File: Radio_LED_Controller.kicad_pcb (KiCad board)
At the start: 2 copper layers, 21.5 x 12.5 mm, 17 parts, among them J1 Conn_01x04_Pin, J2 Conn_01x03_Pin, J3 Conn_01x05, J4 UPDI, J5 Conn_01x02_Pin, J6 Conn_01x02_Pin, J7 Conn_01x05, J8 Conn_01x03_Pin, J9 Conn_01x03_Pin, Q2 SS8050, Q3 SS8050, U1 ATtiny816-M

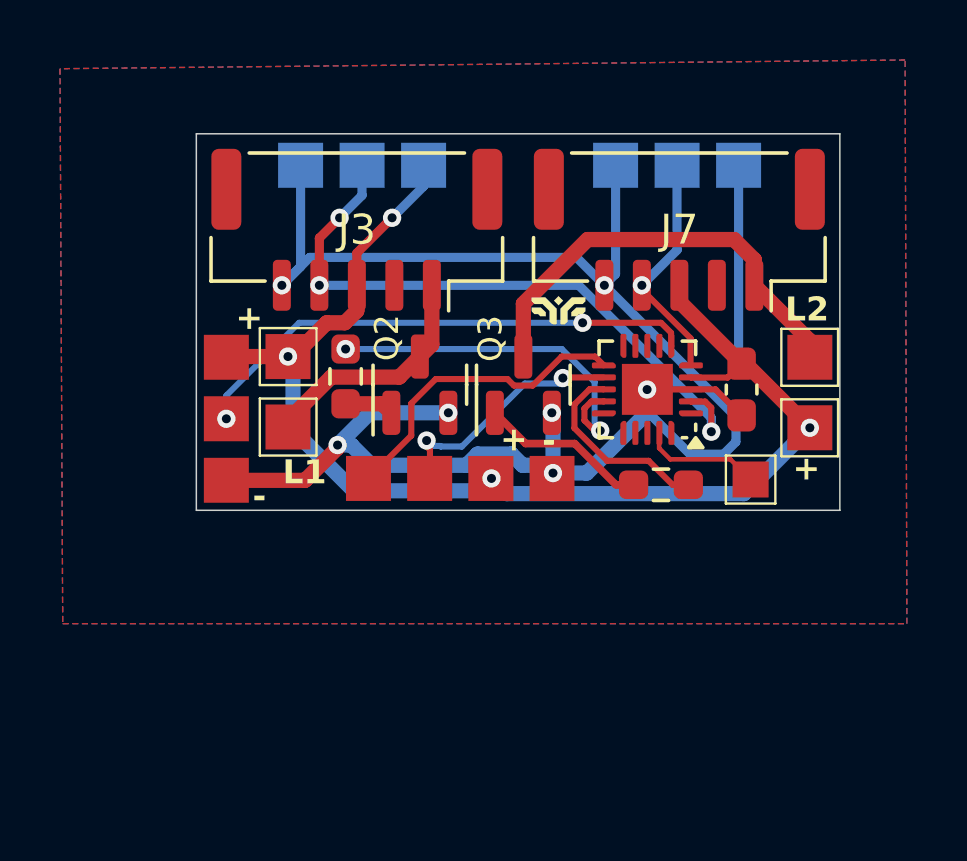
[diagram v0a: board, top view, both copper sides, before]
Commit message: v0.2
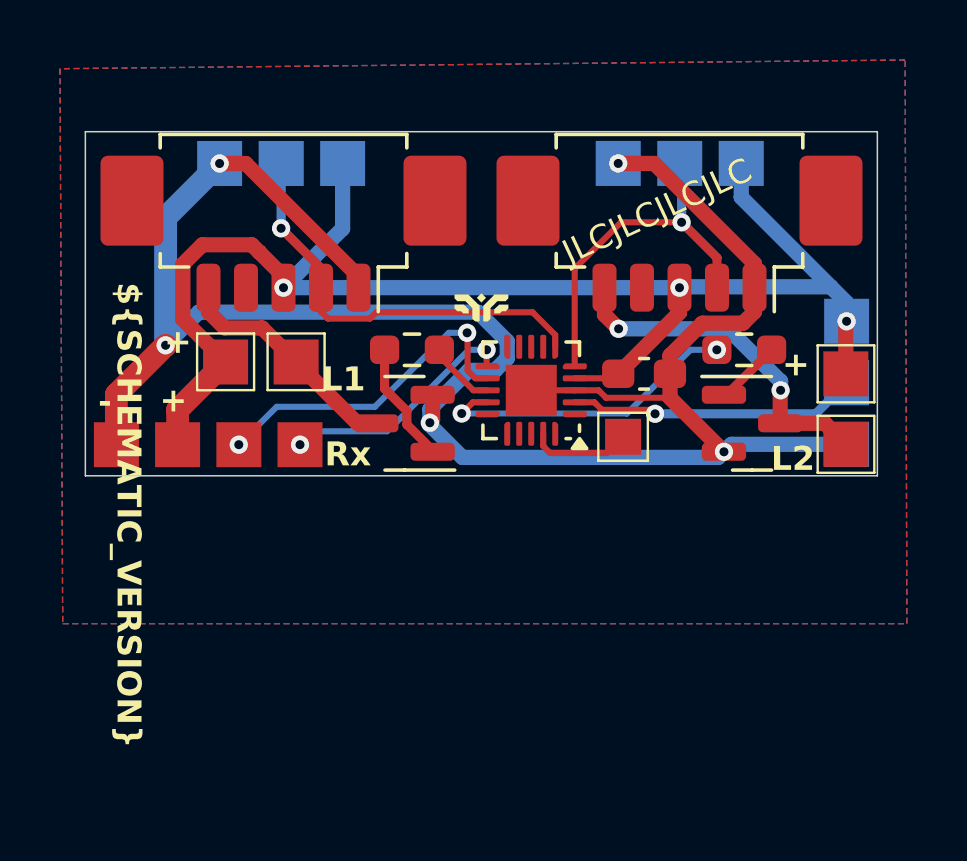
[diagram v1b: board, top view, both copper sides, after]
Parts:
- J2: moved to B.Cu
- J3, J7: footprint Connector_JST:JST_GH_SM05B-GHS-TB_1x05-1MP_P1.25mm_Horizontal -> Connector_Molex:Molex_PicoBlade_53261-0571_1x05-1MP_P1.25mm_Horizontal
- moved J2 22.7 mm to (185.9, 88.7)
- moved Q3 7.73 mm to (181.8, 93.1), turned to 0 degrees
- moved R3 5.29 mm to (181.5, 90.7), turned to 0 degrees
- moved J4 4.48 mm to (177.4, 93.5)
- moved G*** 3.99 mm to (177.3, 90.2)
- moved U1 3.87 mm to (174.4, 92.0)
- moved C2 3.29 mm to (178.2, 91.5), turned to 0 degrees
- moved J1 3.14 mm to (167.7, 92.8), turned to 180 degrees
- moved J8 2.70 mm to (169.1, 85.4)
- moved G*** 2.57 mm to (172.7, 89.2)
- moved J3 2.49 mm to (166.1, 86.2)
- moved R2 2.38 mm to (170.4, 90.7), turned to 180 degrees
- moved J6 2.20 mm to (185.1, 93.0), turned to 90 degrees
- moved J5 1.82 mm to (165.8, 90.8), turned to 180 degrees
- moved Q2 1.39 mm to (170.2, 93.1), turned to 180 degrees
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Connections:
- J3 pad 1: Net-(J3-Pin_1) -> GND
- J3 pad 2: unconnected-(J3-Pin_2-Pad2) -> RGB1
- J3 pad 4: RGB1 -> unconnected-(J3-Pin_4-Pad4)
- J3 pad 5: GND -> Net-(J3-Pin_5)
- J5 pad 1: Net-(J3-Pin_1) -> Net-(J3-Pin_5)
- J7 pad 1: Net-(J6-Pin_1) -> GND
- J7 pad 2: unconnected-(J7-Pin_2-Pad2) -> RGB2
- J7 pad 4: RGB2 -> unconnected-(J7-Pin_4-Pad4)
- J7 pad 5: GND -> Net-(J6-Pin_1)
- Q2 pad 3: Net-(J3-Pin_1) -> Net-(J3-Pin_5)
- U1 pad 13: LED2 -> LED1
- U1 pad 14: LED1 -> LED2
- U1 pad 2: RGB1 -> RGB3
- U1 pad 6: RGB3 -> RGB1
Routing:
- net GND: track 58.0 -> 69.1 mm, vias 7 -> 5
- net LED1: track 12.3 -> 2.30 mm, vias 2 -> 0
- net Net-(J3-Pin_1): track 8.04 -> 0.00 mm
- net Net-(J3-Pin_5): track 0.00 -> 7.94 mm
- net RGB3: track 17.2 -> 9.65 mm, vias 2 -> 1
- net RGB1: track 21.5 -> 14.2 mm, vias 3 -> 1
- net RGB2: track 7.83 -> 12.1 mm
- net LED2: track 6.56 -> 10.4 mm, vias 0 -> 2
- net Net-(Q3-B): track 5.62 -> 2.21 mm
- net Net-(J6-Pin_1): track 14.6 -> 11.6 mm, vias 0 -> 2
- net Tx: track 8.29 -> 11.2 mm
- net Net-(Q2-B): track 1.65 -> 4.06 mm
- net Rx: track 10.5 -> 8.10 mm, vias 0 -> 2
- net VCC: track 50.9 -> 48.9 mm, vias 4 -> 3
- net Net-(J4-Pin_1): track 3.98 -> 3.39 mm
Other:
- board size 21.5 x 12.5 mm -> 26.4 x 11.5 mm
- board text added: "${SCHEMATIC_VERSION}"
- board text added: "JLCJLCJLCJLC"
- board text added: "^"
